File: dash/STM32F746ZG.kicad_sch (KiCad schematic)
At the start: 84 parts, among them J1 SHF10501LDTHLC, J2 XF2M-4015-1A, J3 USB_C_Receptacle_USB2.0_16P, J4 MEM2061-01-188-00-A, SW1 KMR221G LFS, SW2 SW_SPST, SW3 KMR221G LFS, U1 STM32F746ZGTx, U2 W9812G6KH-5, U3 XPT2046TS, Y1 25MHz

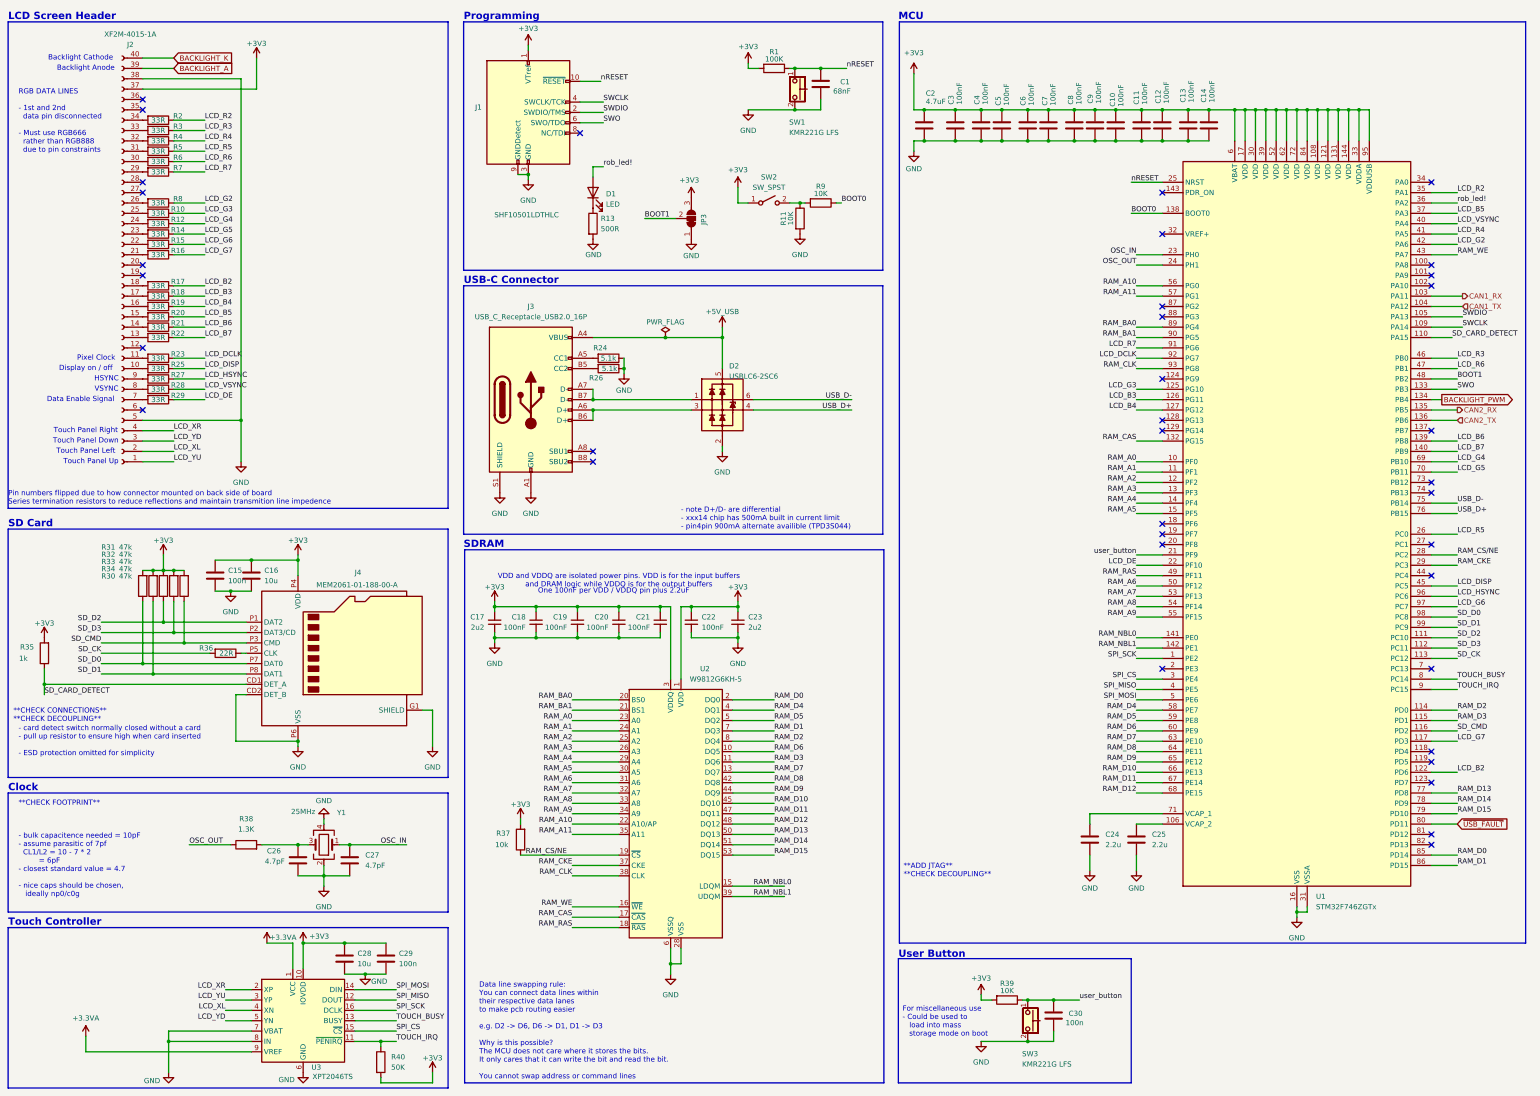
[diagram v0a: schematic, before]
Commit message: Adding silkscreen, cleaning up DRC
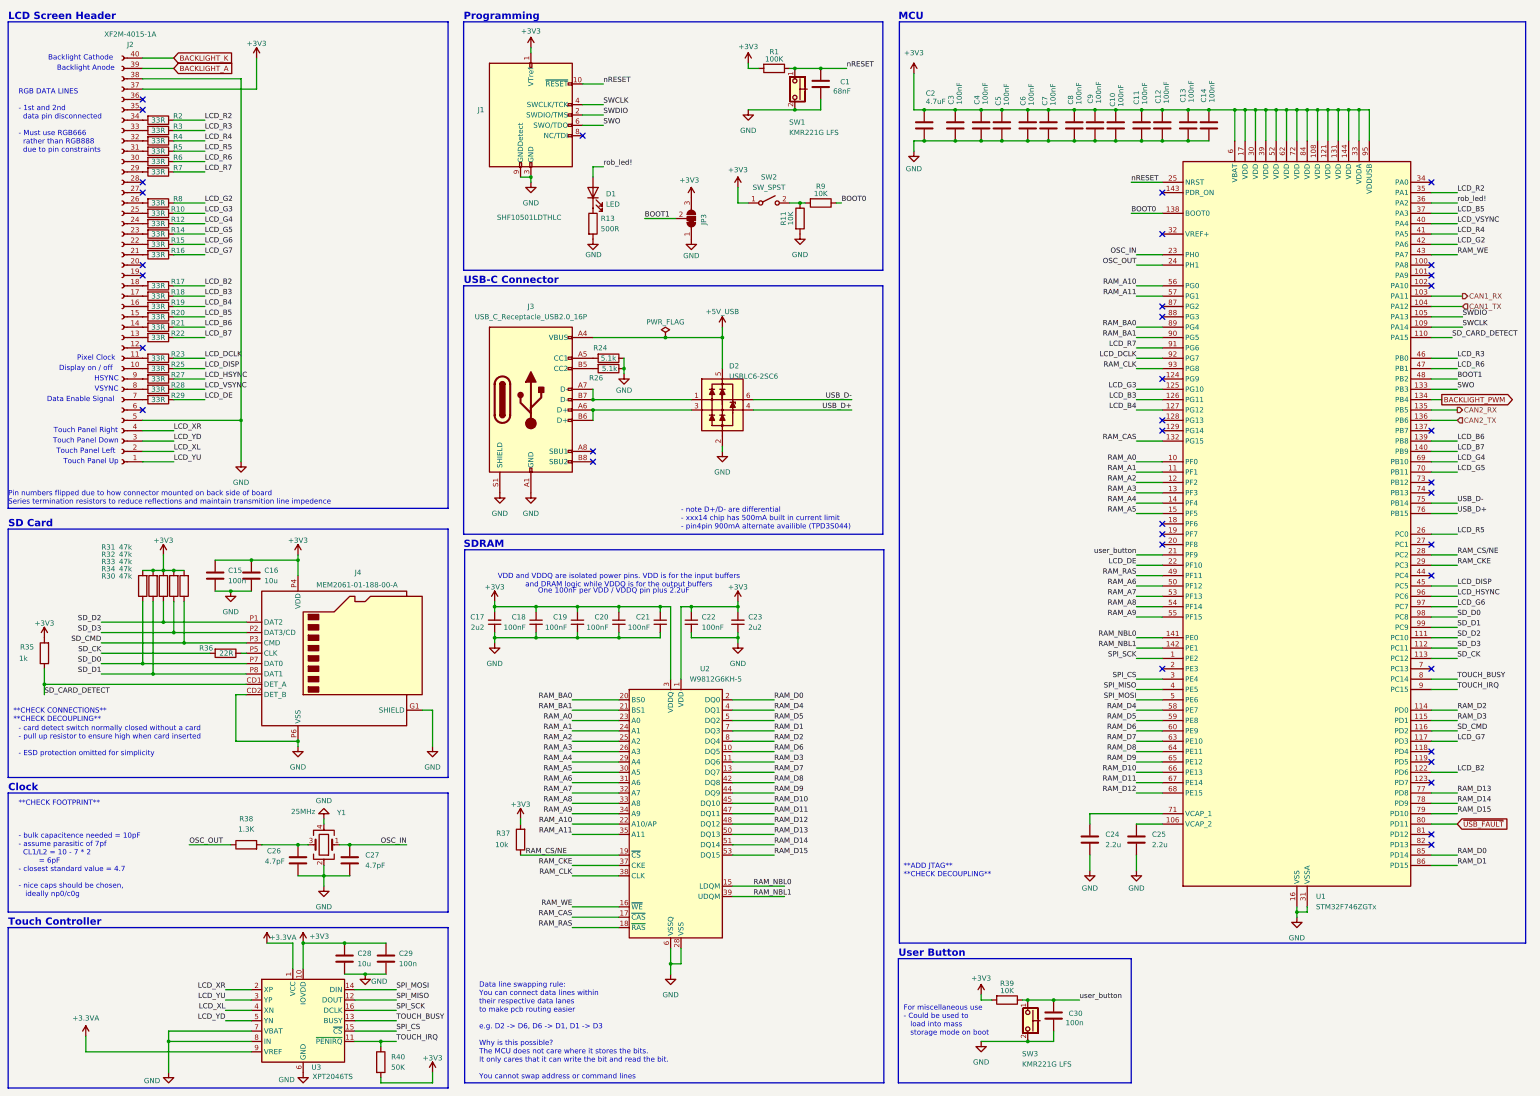
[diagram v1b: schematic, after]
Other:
- moved on the sheet: J1
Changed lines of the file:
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@@
 	(text "For miscellaneous use\n- Could be used to\n   load into mass\n   storage mode on boot"
 		(exclude_from_sim no)
-		(at 241.046 268.224 0)
+		(at 241.3 267.97 0)
 		(effects
 			(font
@@
 	(text "User Button"
 		(exclude_from_sim no)
-		(at 240.03 251.714 0)
+		(at 240.03 251.46 0)
 		(effects
 			(font
@@
 	)
 	(junction
-		(at 149.225 60.325)
+		(at 149.86 60.96)
 		(diameter 0)
 		(color 0 0 0 0)
@@
 	)
 	(no_connect
-		(at 161.925 50.165)
+		(at 162.56 50.8)
 	)
 	(no_connect
@@
 	(wire
 		(pts
-			(xy 167.64 45.085) (xy 161.925 45.085)
+			(xy 167.64 45.72) (xy 162.56 45.72)
 		)
 		(stroke
@@
 	(wire
 		(pts
-			(xy 167.64 42.545) (xy 161.925 42.545)
+			(xy 167.64 43.18) (xy 162.56 43.18)
 		)
 		(stroke
@@
 	(wire
 		(pts
-			(xy 149.225 60.325) (xy 149.225 61.595)
+			(xy 149.86 60.96) (xy 149.86 62.23)
 		)
 		(stroke
@@
 	(wire
 		(pts
-			(xy 146.685 60.325) (xy 149.225 60.325)
+			(xy 147.32 60.96) (xy 149.86 60.96)
 		)
 		(stroke
@@
 	(wire
 		(pts
-			(xy 167.005 37.465) (xy 161.925 37.465)
+			(xy 167.64 38.1) (xy 162.56 38.1)
 		)
 		(stroke
@@
 	(wire
 		(pts
-			(xy 149.225 29.845) (xy 149.225 28.575)
+			(xy 149.86 30.48) (xy 149.86 29.21)
 		)
 		(stroke
@@
 	(wire
 		(pts
-			(xy 167.64 47.625) (xy 161.925 47.625)
+			(xy 167.64 48.26) (xy 162.56 48.26)
 		)
 		(stroke
@@
 	)
 	(label "SWCLK"
-		(at 167.64 42.545 0)
+		(at 167.64 43.18 0)
 		(effects
 			(font
@@
 	)
 	(label "SWDIO"
-		(at 167.64 45.085 0)
+		(at 167.64 45.72 0)
 		(effects
 			(font
@@
 	)
 	(label "nRESET"
-		(at 167.005 37.465 0)
+		(at 167.64 38.1 0)
 		(effects
 			(font
@@
 	)
 	(label "SWO"
-		(at 167.64 47.625 0)
+		(at 167.64 48.26 0)
 		(effects
 			(font
@@
 		(length 2.54)
 		(shape round)
-		(at 80.645 50.165 270)
+		(at 80.645 50.8 270)
 		(fields_autoplaced yes)
 		(effects
@@
 		)
 		(property "Netclass" "LCD"
-			(at 83.185 49.5554 90)
+			(at 83.185 50.1904 90)
 			(effects
 				(font
@@
 		)
 		(property "Component Class" ""
-			(at -168.91 -90.17 0)
+			(at -168.91 -89.535 0)
 			(effects
 				(font
@@
 	(symbol
 		(lib_id "power:+3V3")
-		(at 149.225 28.575 0)
+		(at 149.86 29.21 0)
 		(unit 1)
 		(exclude_from_sim no)
@@
 		(dnp no)
 		(property "Reference" "#PWR03"
-			(at 149.225 32.385 0)
+			(at 149.86 33.02 0)
 			(effects
 				(font
@@
 		)
 		(property "Value" "+3V3"
-			(at 149.225 24.511 0)
+			(at 149.86 25.146 0)
 			(effects
 				(font
@@
 		)
 		(property "Footprint" ""
-			(at 149.225 28.575 0)
+			(at 149.86 29.21 0)
 			(effects
 				(font
@@
 		)
 		(property "Datasheet" ""
-			(at 149.225 28.575 0)
+			(at 149.86 29.21 0)
 			(effects
 				(font
@@
 		)
 		(property "Description" "Power symbol creates a global label with name \"+3V3\""
-			(at 149.225 28.575 0)
+			(at 149.86 29.21 0)
 			(effects
 				(font
@@
 	(symbol
 		(lib_id "Connector:Conn_ARM_JTAG_SWD_10")
-		(at 149.225 45.085 0)
+		(at 149.86 45.72 0)
 		(unit 1)
 		(exclude_from_sim no)
@@
 		(dnp no)
 		(property "Reference" "J1"
-			(at 137.795 43.8149 0)
+			(at 138.43 44.4499 0)
 			(effects
 				(font
@@
 		)
 		(property "Value" "SHF10501LDTHLC"
-			(at 156.718 70.231 0)
+			(at 157.353 70.866 0)
 			(effects
 				(font
@@
 		)
 		(property "Footprint" "SUFST:SHF10501LDSMLC"
-			(at 149.225 45.085 0)
+			(at 149.86 45.72 0)
 			(effects
 				(font
@@
 		)
 		(property "Datasheet" "http://infocenter.arm.com/help/topic/com.arm.doc.ddi0314h/DDI0314H_coresight_components_trm.pdf"
-			(at 140.335 76.835 90)
+			(at 140.97 77.47 90)
 			(effects
 				(font
@@
 		)
 		(property "Description" "Cortex Debug Connector, standard ARM Cortex-M SWD and JTAG interface"
-			(at 149.225 45.085 0)
+			(at 149.86 45.72 0)
 			(effects
 				(font
@@
 	(symbol
 		(lib_id "power:GND")
-		(at 149.225 61.595 0)
+		(at 149.86 62.23 0)
 		(mirror y)
 		(unit 1)
@@
 		(fields_autoplaced yes)
 		(property "Reference" "#PWR09"
-			(at 149.225 67.945 0)
+			(at 149.86 68.58 0)
 			(effects
 				(font
@@
 		)
 		(property "Value" "GND"
-			(at 149.225 66.675 0)
+			(at 149.86 67.31 0)
 			(effects
 				(font
@@
 		)
 		(property "Footprint" ""
-			(at 149.225 61.595 0)
+			(at 149.86 62.23 0)
 			(effects
 				(font
@@
 		)
 		(property "Datasheet" ""
-			(at 149.225 61.595 0)
+			(at 149.86 62.23 0)
 			(effects
 				(font
@@
 		)
 		(property "Description" "Power symbol creates a global label with name \"GND\" , ground"
-			(at 149.225 61.595 0)
+			(at 149.86 62.23 0)
 			(effects
 				(font
